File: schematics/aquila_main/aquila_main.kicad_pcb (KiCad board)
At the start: 4 copper layers, 98 x 98 mm, 132 parts, among them IC1 MS5611-01BA03, J1 120591-1, J10 PYRO_3, J11 PYRO_2, J12 PYRO_4, J13 AudioJack3_SwitchTR, J14 SERVO, J2 1043P, J3 1043P, J4 PWR, J5 TELEM, J6 GPS, J7 BARO, J8 BMI-S-201, J9 PYRO_1, Q1 IRF7509PbF, Q2 IRF7509PbF, Q3 IRF7509PbF, Q4 IRF7509PbF, U1 LM2576S-3.3/NOPB, U2 LM2576D2TR4-5G, U3 MAX-M8Q, U4 Si4463, U5 B3520, U6 SKY65723-11, U7 ADXL357, U8 BQ29200, U9 Teensy4.1, Y1 30M

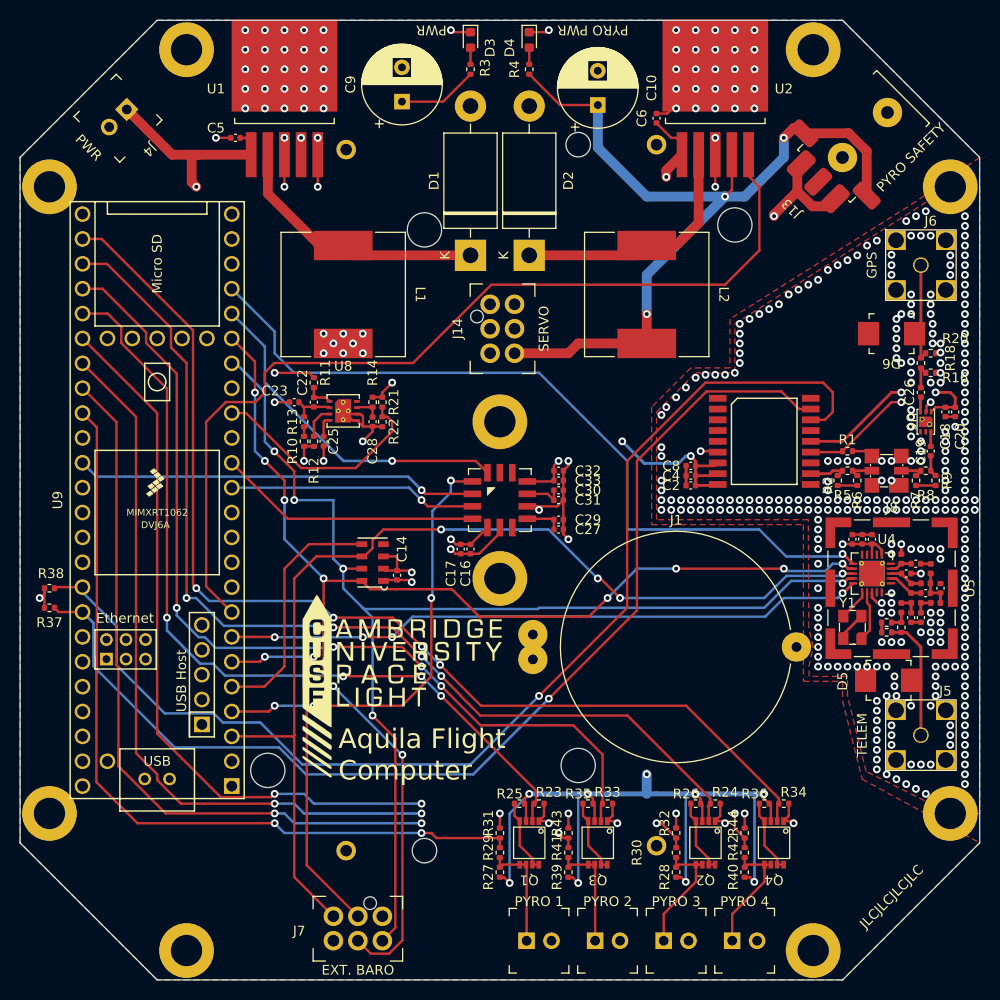
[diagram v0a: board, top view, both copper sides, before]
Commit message: minor adjustments
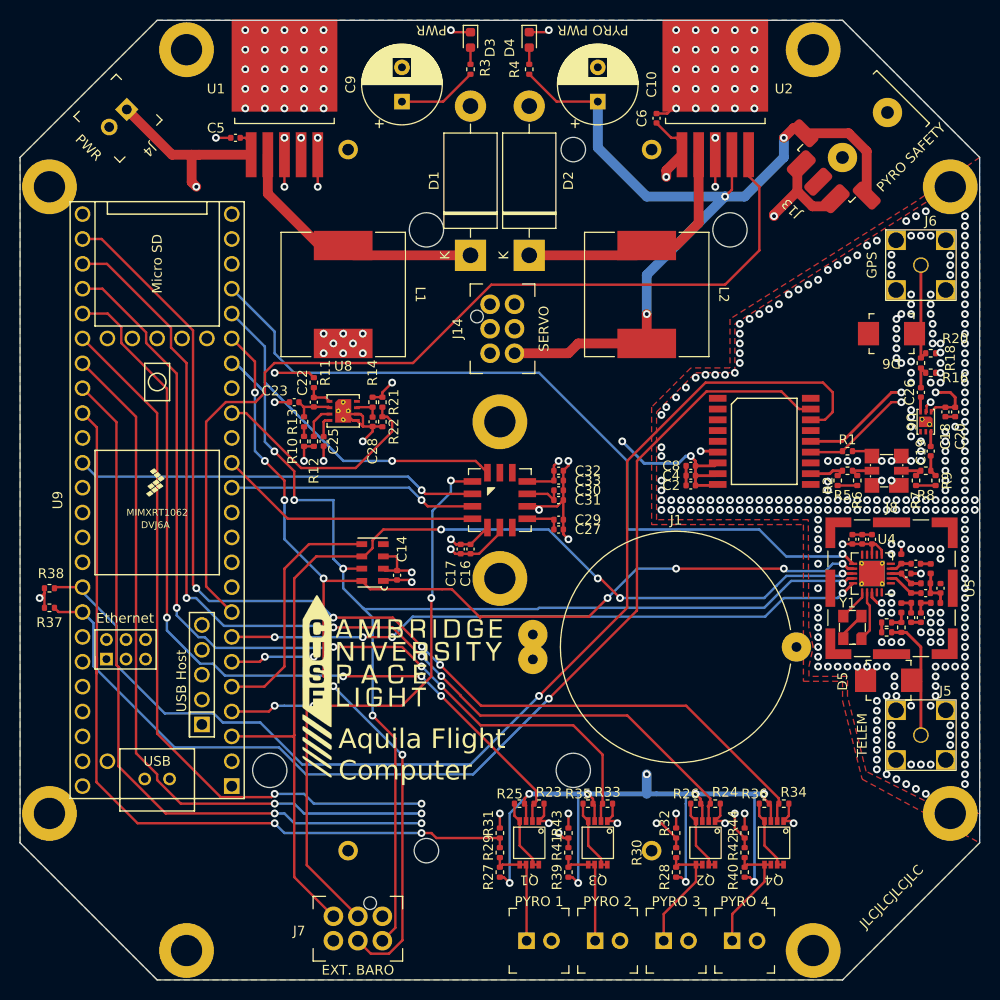
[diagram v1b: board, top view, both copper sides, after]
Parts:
- moved J2 0.71 mm to (165.5, 100.0)
- moved C10 0.35 mm to (160.0, 59.3)
- moved J3 0.20 mm to (134.5, 100.0)
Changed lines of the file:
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@@
   )
   (footprint "Capacitor_THT:CP_Radial_D8.0mm_P3.50mm" (layer "F.Cu")
-    (at 160 59.652651 90)
+    (at 160 59.3 90)
     (descr "CP, Radial series, Radial, pin pitch=3.50mm, , diameter=8mm, Electrolytic Capacitor")
     (tags "CP Radial series Radial pin pitch 3.50mm  diameter 8mm Electrolytic Capacitor")
@@
   )
   (footprint "aquila:1043" (layer "B.Cu")
-    (at 166 99.5 90)
+    (at 165.5 100 90)
     (property "DigiKey" "36-1043P-ND")
     (property "Sheetfile" "aquila_main.kicad_sch")
@@
   )
   (footprint "aquila:1043" (layer "B.Cu")
-    (at 134.3 100 -90)
+    (at 134.5 100 -90)
     (property "DigiKey" "36-1043P-ND")
     (property "Sheetfile" "aquila_main.kicad_sch")
@@
   (segment (start 179 63) (end 180 62) (width 1) (layer "F.Cu") (net 4))
   (segment (start 180.564971 62) (end 181.100505 62.535534) (width 1) (layer "F.Cu") (net 4))
-  (segment (start 160 59.652651) (end 156.142651 59.652651) (width 0.25) (layer "F.Cu") (net 4))
+  (segment (start 155.79 59.3) (end 160 59.3) (width 0.25) (layer "F.Cu") (net 4))
   (segment (start 157 85) (end 151.5 85) (width 1) (layer "F.Cu") (net 4))
   (segment (start 173.7 68.3) (end 173.7 64.725) (width 0.25) (layer "F.Cu") (net 4))
-  (segment (start 156.142651 59.652651) (end 153 56.51) (width 0.25) (layer "F.Cu") (net 4))
   (segment (start 158 84) (end 157 85) (width 1) (layer "F.Cu") (net 4))
   (segment (start 181.100505 62.899495) (end 181.100505 62.535534) (width 0.25) (layer "F.Cu") (net 4))
@@
   (segment (start 187.464466 64.374703) (end 187.464466 68.899495) (width 1) (layer "F.Cu") (net 4))
   (segment (start 173 69) (end 173.7 68.3) (width 0.25) (layer "F.Cu") (net 4))
+  (segment (start 153 56.51) (end 155.79 59.3) (width 0.25) (layer "F.Cu") (net 4))
   (segment (start 165 84) (end 165 81) (width 1) (layer "F.Cu") (net 4))
   (segment (start 165 84) (end 158 84) (width 1) (layer "F.Cu") (net 4))
@@
   (segment (start 173 69) (end 165 69) (width 1) (layer "B.Cu") (net 4))
   (segment (start 175 69) (end 179 65) (width 1) (layer "B.Cu") (net 4))
-  (segment (start 160 64) (end 160 59.652651) (width 1) (layer "B.Cu") (net 4))
   (segment (start 173 69) (end 175 69) (width 1) (layer "B.Cu") (net 4))
   (segment (start 179 65) (end 179 63) (width 1) (layer "B.Cu") (net 4))
+  (segment (start 160 64) (end 160 59.3) (width 1) (layer "B.Cu") (net 4))
   (segment (start 165 69) (end 160 64) (width 1) (layer "B.Cu") (net 4))
   (segment (start 165 77) (end 173 69) (width 1) (layer "B.Cu") (net 4))
